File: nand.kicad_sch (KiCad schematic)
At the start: 2 parts, among them U1 MCIMX6Y2DVM09AB

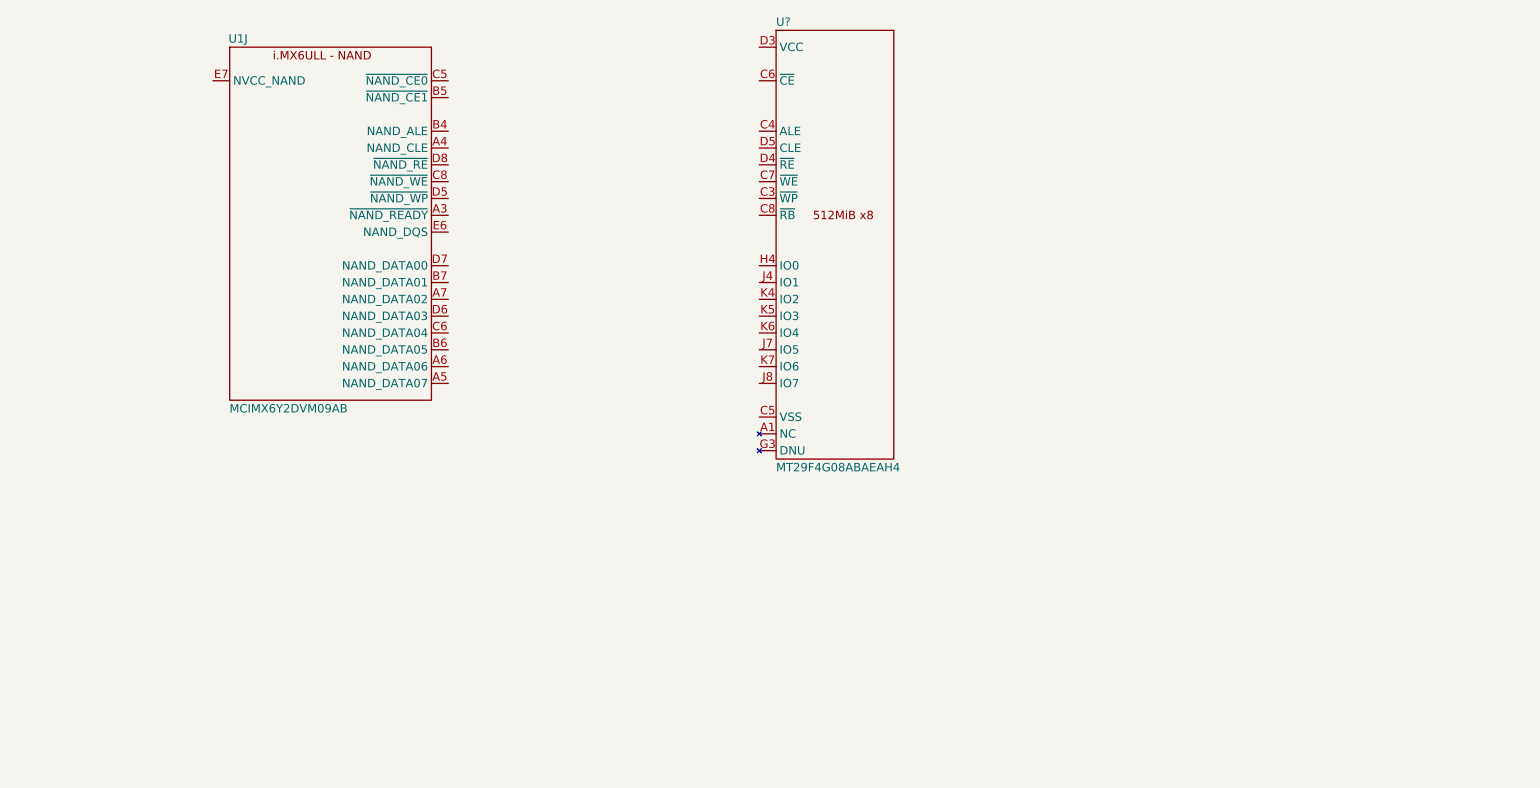
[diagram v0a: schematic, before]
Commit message: NAND
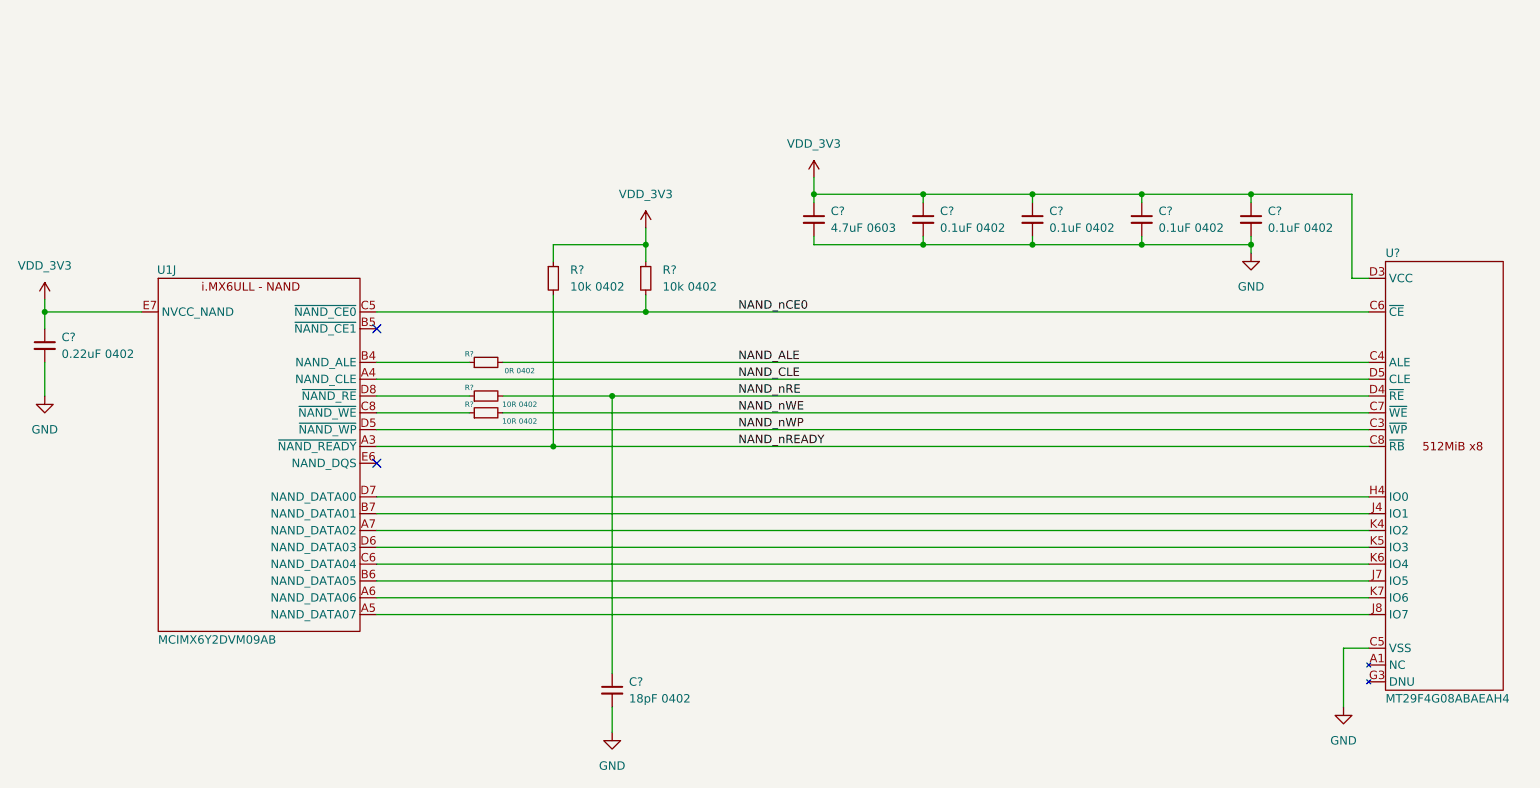
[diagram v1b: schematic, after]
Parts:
- added C?: 18pF 0402, symbol Device:C_Small
- added C? (x4): 0.1uF 0402, symbol Device:C_Small
- added C?: 0.22uF 0402, symbol Device:C_Small
- added C?: 4.7uF 0603, symbol Device:C_Small
- added R? (x2): 10k 0402, symbol Device:R_Small
- added R? (x2): 10R 0402, symbol Device:R_Small
- added R?: 0R 0402, symbol Device:R_Small
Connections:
- net VCC: now also U1.E7 (NVCC_NAND), C?.1, C?.1, C?.1, C?.1, C?.1, C?.1, R?.1, R?.1
- net NAND_nREADY: now reaches U1.A3 (~{NAND_READY})
- net NAND_nREADY: now also U?.C8 (~{RB}), R?.2
- net NAND_CLE: now reaches U1.A4 (NAND_CLE)
- net NAND_CLE: now also U?.D5 (CLE)
- net at U1.A5 (NAND_DATA07): now also U?.J8 (IO7)
- net at U1.A6 (NAND_DATA06): now also U?.K7 (IO6)
- net at U1.A7 (NAND_DATA02): now also U?.K4 (IO2)
- net at U1.B4 (NAND_ALE): now also R?.1
- net at U1.B6 (NAND_DATA05): now also U?.J7 (IO5)
- net at U1.B7 (NAND_DATA01): now also U?.J4 (IO1)
- net NAND_nCE0: now reaches U1.C5 (~{NAND_CE0})
- net NAND_nCE0: now also U?.C6 (~{CE}), R?.2
- net at U1.C6 (NAND_DATA04): now also U?.K6 (IO4)
- net at U1.C8 (~{NAND_WE}): now also R?.1
- net NAND_nWP: now reaches U1.D5 (~{NAND_WP})
- net NAND_nWP: now also U?.C3 (~{WP})
- net at U1.D6 (NAND_DATA03): now also U?.K5 (IO3)
- net at U1.D7 (NAND_DATA00): now also U?.H4 (IO0)
- net at U1.D8 (~{NAND_RE}): now also R?.1
- net NAND_ALE: now reaches U?.C4 (ALE)
- net NAND_ALE: now also R?.2
- net NAND_nWE: now reaches U?.C7 (~{WE})
- net NAND_nWE: now also R?.2
- net NAND_nRE: now reaches U?.D4 (~{RE})
- net NAND_nRE: now also C?.1, R?.2
- net VSS renamed GND
- net GND: now also C?.2, C?.2, C?.2, C?.2, C?.2, C?.2, C?.2
- no-connect marks 0 -> 2
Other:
- moved on the sheet: U1J, U?
